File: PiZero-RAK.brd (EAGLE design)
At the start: 104.8 x 54.6 mm, 39 parts, among them IC1 PCF8523, J1 CON_HEADER_1X05-PTH, J11 CON_HEADER_1X06-PTH, J2 CONN_20X2HLE, J3 CON_HEADER_1X05-PTH, J4 CON_HEADER_1X05-PTH, Q1 CJ2302, X1 SPTAF_23.5, X2 SPTAF_25.0MM, Y1 32.768KHz

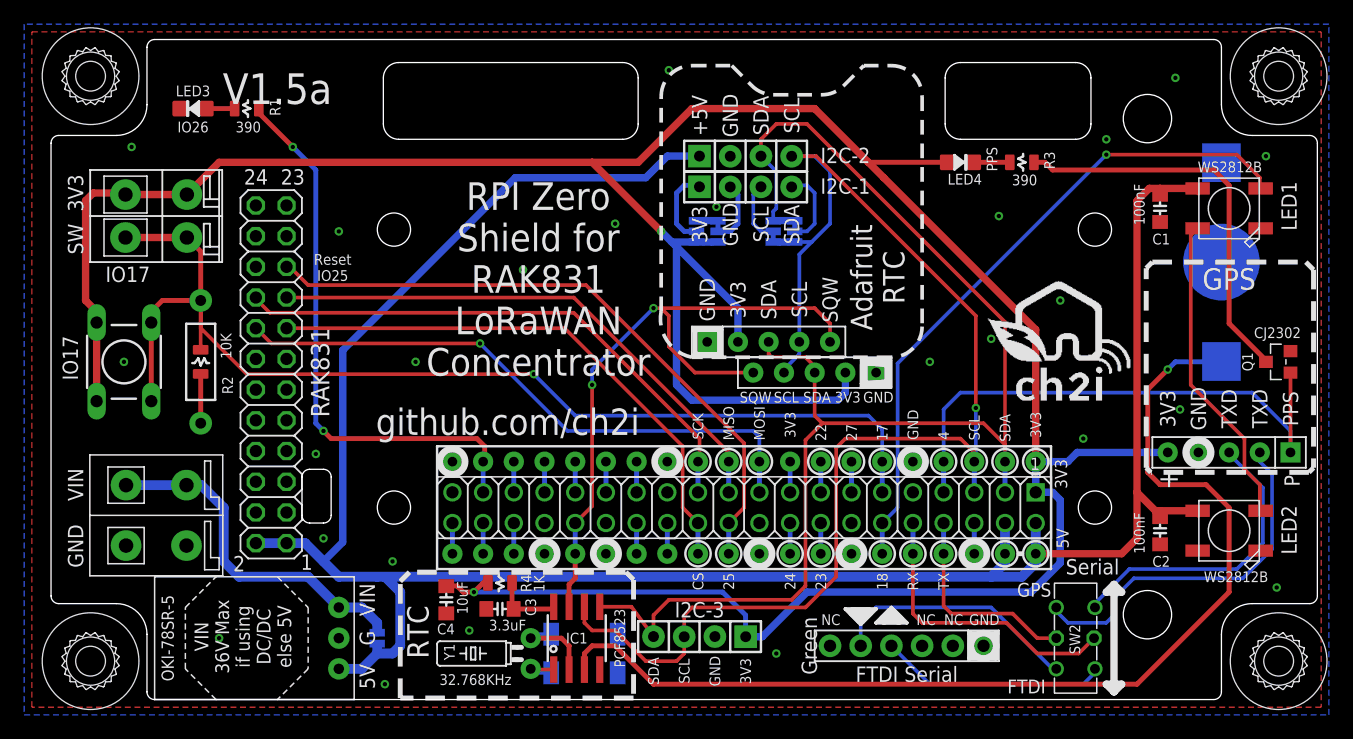
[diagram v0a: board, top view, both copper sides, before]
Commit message: My version
Change 10cm Max
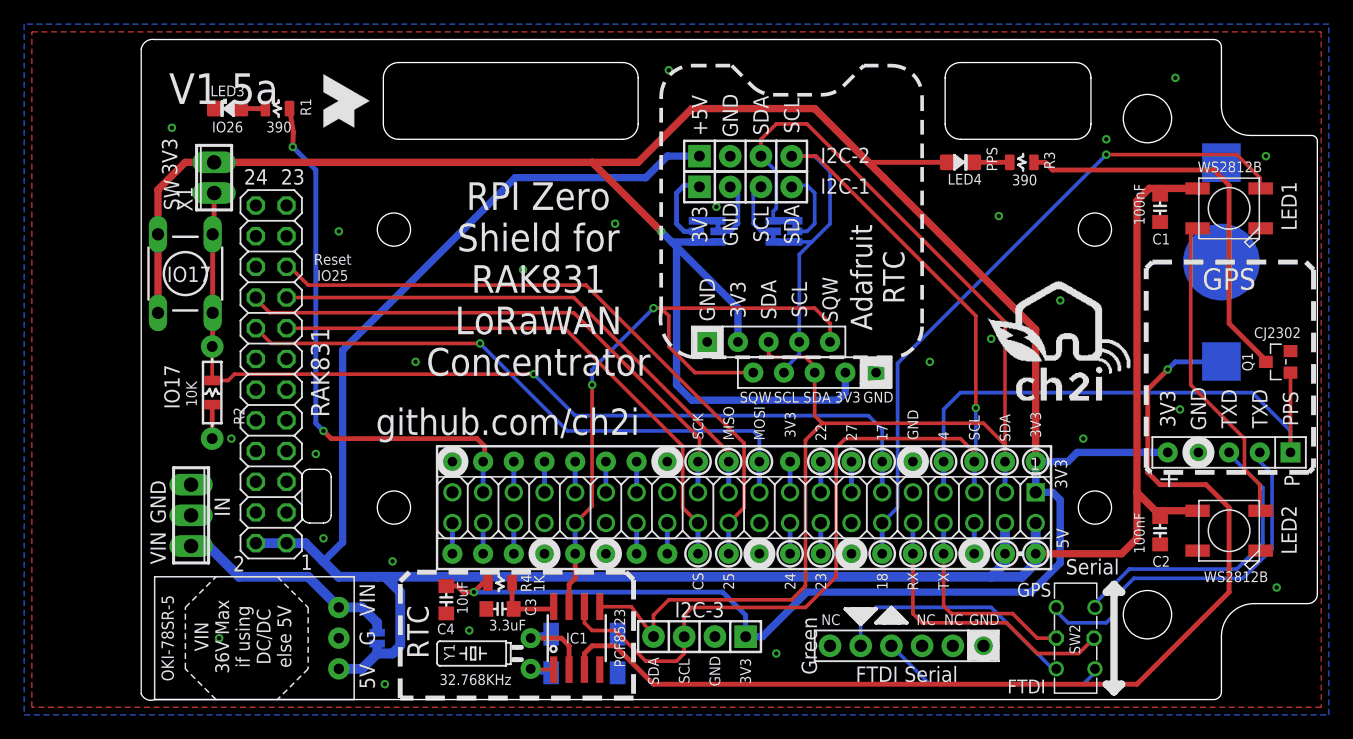
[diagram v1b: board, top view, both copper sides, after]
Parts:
- removed U$10: (no value), _c2h:ENCLOSURE_1591B
- removed X2: SPTAF_25.0MM, _c2h:SPTAF_2X50
- added IN: (no value), con-phoenix-254:3POL254
- added U$6, U$7: (no value), ricaun:RICAUN
- R2: device _c2h:AXIAL-0.4 -> _c2h:AXIAL-0.3
- X1: value SPTAF_23.5 -> (none); device _c2h:FFKV2_35 -> con-phoenix-254:2POL254
- moved S1 8.90 mm to (20.3, 41.6)
- moved X1 5.33 mm to (22.7, 49.5)
- moved LED3 2.86 mm to (23.8, 55.2)
- moved R105 2.71 mm to (22.5, 31.8)
- moved R2 2.71 mm to (22.5, 31.8)
- moved R1 2.54 mm to (27.9, 55.2)
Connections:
- net 3V3: no longer X1.2A
- net GND: now also IN.1, IN.2; no longer X2.1, X2.1A
- net GPIO17: no longer X1.1A
- net VIN: now also IN.3; no longer X2.2, X2.2A
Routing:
- net GPIO17: track 94.3 -> 78.8 mm
- net 3V3: track 254.9 -> 241.7 mm
- net VIN: track 30.0 -> 18.8 mm
- net GND: track 8.40 -> 7.13 mm
- net GPIO26: track 46.6 -> 45.5 mm
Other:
- board size 104.8 x 54.6 mm -> 97.3 x 54.7 mm
